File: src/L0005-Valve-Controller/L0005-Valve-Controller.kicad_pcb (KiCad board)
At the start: 4 copper layers, 141.7 x 50.5 mm, 103 parts, among them J1 Jumper_NO, K1 AQH0223AX, K2 AQH0223AX, K3 AQH0223AX, K4 AQH0223AX, K5 AQH0223AX, K6 AQH0223AX, P1 3220-20-0200-00, P10 353620650, P11 353620650, P12 353620650, P13 353620650, P14 647676-3, P15 647676-3, P16 647676-2, P2 140-504-415-000, P3 647676-3, P4 647676-3, P5 647676-3, P6 647676-3, P7 647676-3, P8 647676-3, P9 647676-2, Q1 CMLDM7003, Q2 CMLDM7003, U1 STM32H750VBTx, U2 LMS8117AMP-3.3_NOPB, U3 MAX3370EXK+T, U4 MAX3370EXK+T, U5 Optocoupler

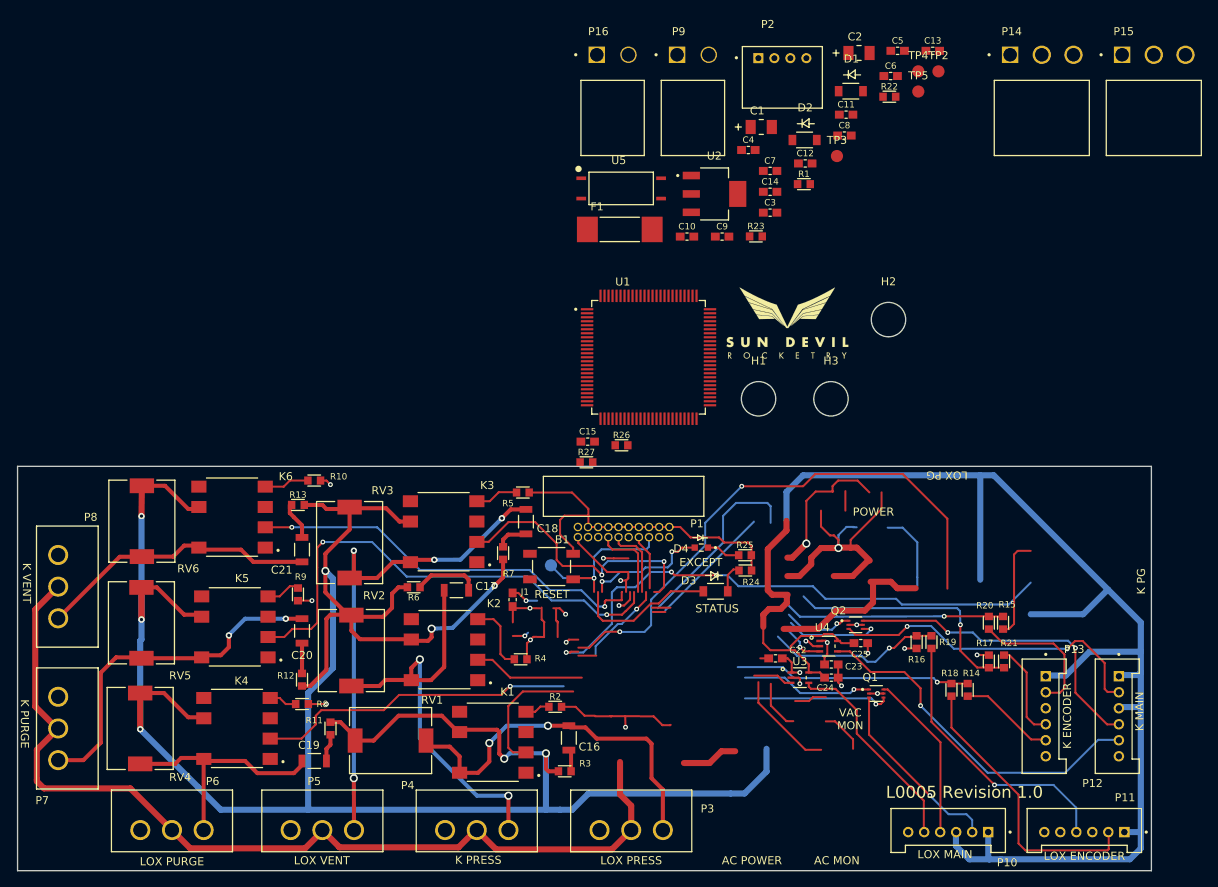
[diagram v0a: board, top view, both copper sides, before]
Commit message: routed rev 2
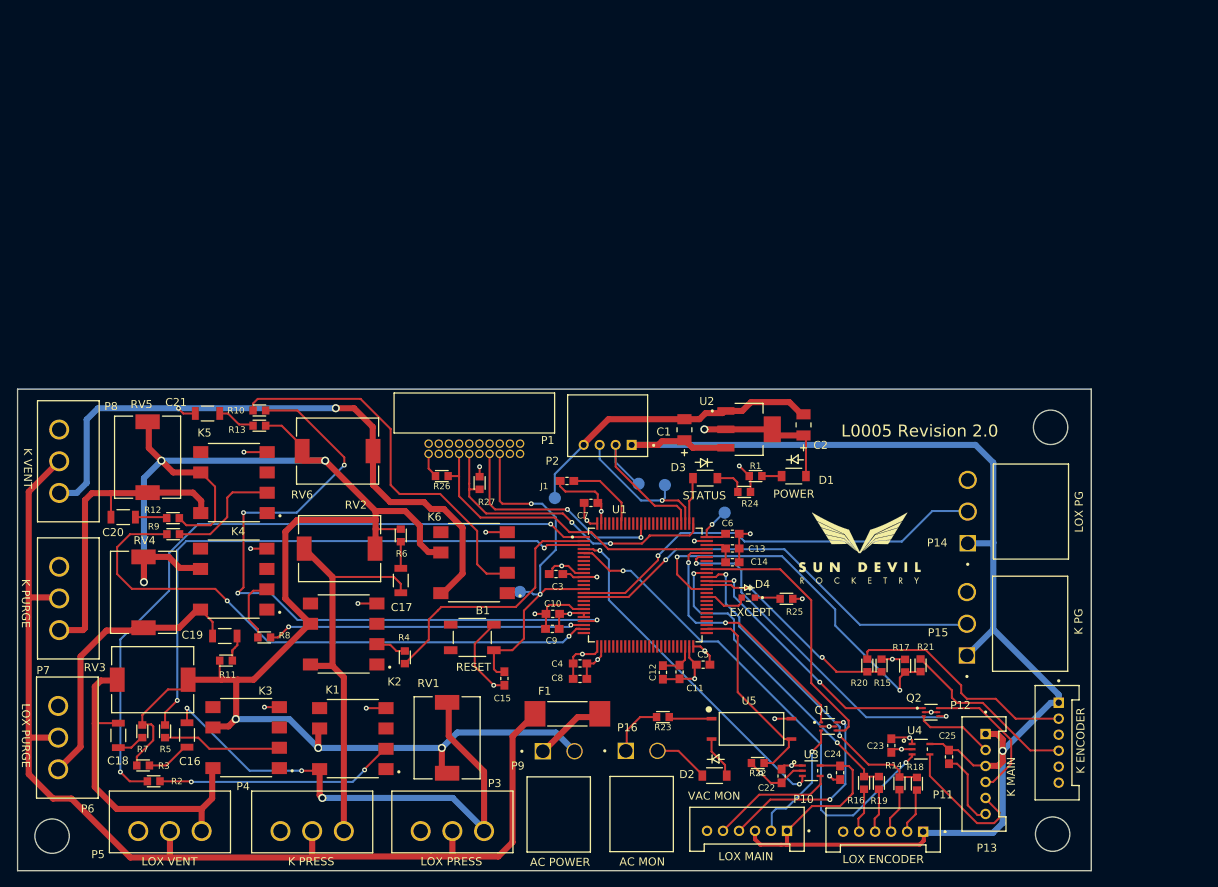
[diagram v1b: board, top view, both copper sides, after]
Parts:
- TP2, TP3, TP4, TP5: moved to B.Cu
- moved H3 111.7 mm to (61.2, 123.2)
- moved P9 88.7 mm to (122.6, 112.6)
- moved P16 87.1 mm to (132.9, 112.5)
- moved R22 84.9 mm to (149.4, 114.0), turned to 180 degrees
- moved C5 80.5 mm to (142.6, 101.8)
- moved D2 80.2 mm to (144.0, 115.6)
- moved P15 77.5 mm to (175.6, 100.6), turned to 90 degrees
- moved C8 75.5 mm to (127.2, 103.5)
- moved C11 72.7 mm to (139.6, 102.7), turned to 90 degrees
- moved TP2 71.7 mm to (124.1, 80.9), turned to 180 degrees
- moved U5 69.5 mm to (148.6, 109.8)
- moved C4 67.5 mm to (127.2, 101.6)
- moved H2 67.5 mm to (186.3, 122.9)
- moved C13 67.1 mm to (146.3, 87.2), turned to 180 degrees
- moved C12 66.1 mm to (137.6, 102.7), turned to 90 degrees
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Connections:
- C11 pad 1: Net-(C11-Pad1) -> Earth
- C12 pad 1: Net-(C11-Pad1) -> Earth
- C13 pad 1: Net-(C11-Pad1) -> Earth
- C14 pad 1: Net-(C11-Pad1) -> Earth
- U1 pad 60: unconnected-(U1-Pad60) -> EXECPT
- U1 pad 68: RX -> unconnected-(U1-Pad68)
- U1 pad 69: TX -> unconnected-(U1-Pad69)
- U1 pad 78: EXECPT -> TX
- U1 pad 79: unconnected-(U1-Pad79) -> RX
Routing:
- net SOL1: track 0.00 -> 87.3 mm, vias 0 -> 2
- net SOL4: track 0.00 -> 86.6 mm, vias 0 -> 4
- net AC_NEUTRAL: track 308.9 -> 223.6 mm, vias 8 -> 6
- net SOL3: track 0.00 -> 74.3 mm, vias 0 -> 2
- net SOL6: track 0.00 -> 72.3 mm, vias 0 -> 2
- net SBV2_PUL: track 5.66 -> 62.7 mm, vias 1 -> 2
- net Net-(K5-Pad2): track 63.7 -> 14.7 mm, vias 3 -> 0
- net Net-(C21-Pad2): track 35.0 -> 81.4 mm, vias 0 -> 2
- net Net-(K4-Pad2): track 52.9 -> 8.43 mm, vias 3 -> 0
- net SBV1_PUL: track 4.98 -> 42.7 mm, vias 0 -> 2
- net SOL5: track 3.28 -> 39.7 mm, vias 0 -> 2
- net SOL2: track 0.00 -> 32.6 mm
- net SBV2_EN: track 12.0 -> 43.9 mm, vias 1 -> 2
- net Net-(P12-Pad2): track 40.6 -> 9.69 mm, vias 2 -> 0
- net Net-(P11-Pad2): track 35.7 -> 5.62 mm
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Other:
- board size 141.7 x 50.5 mm -> 134.2 x 60.2 mm
- board text added: "L0005 Revision 2.0"
- board text removed: "L0005 Revision 1.0"
